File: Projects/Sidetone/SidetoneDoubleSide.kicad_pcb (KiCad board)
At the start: 2 copper layers, 109.1 x 105 mm, 54 parts, among them Q1 2N3904, Q2 2N3904, Q3 2N3904, SW1 morse key, SW2 On/off, U1 4N35, U2 LM324, U3 LM386

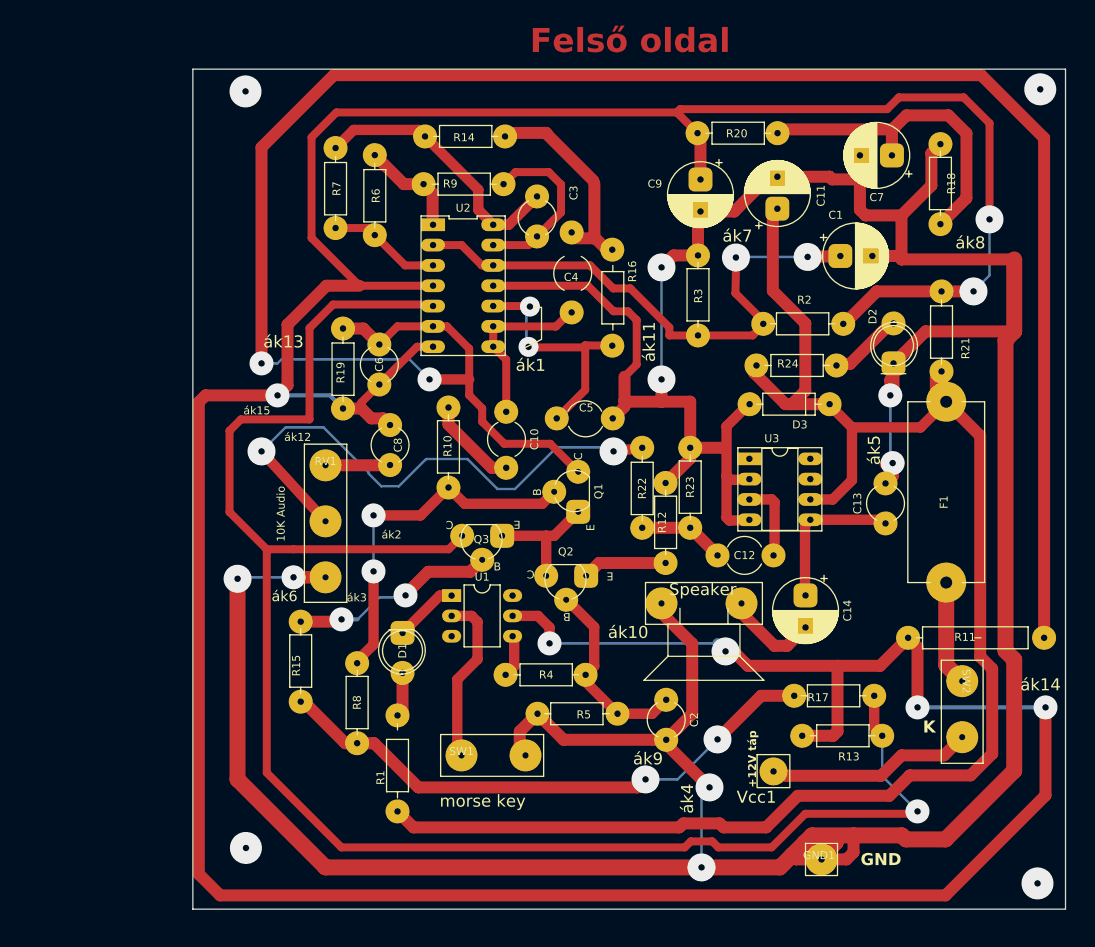
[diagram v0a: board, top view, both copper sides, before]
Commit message: 20240226
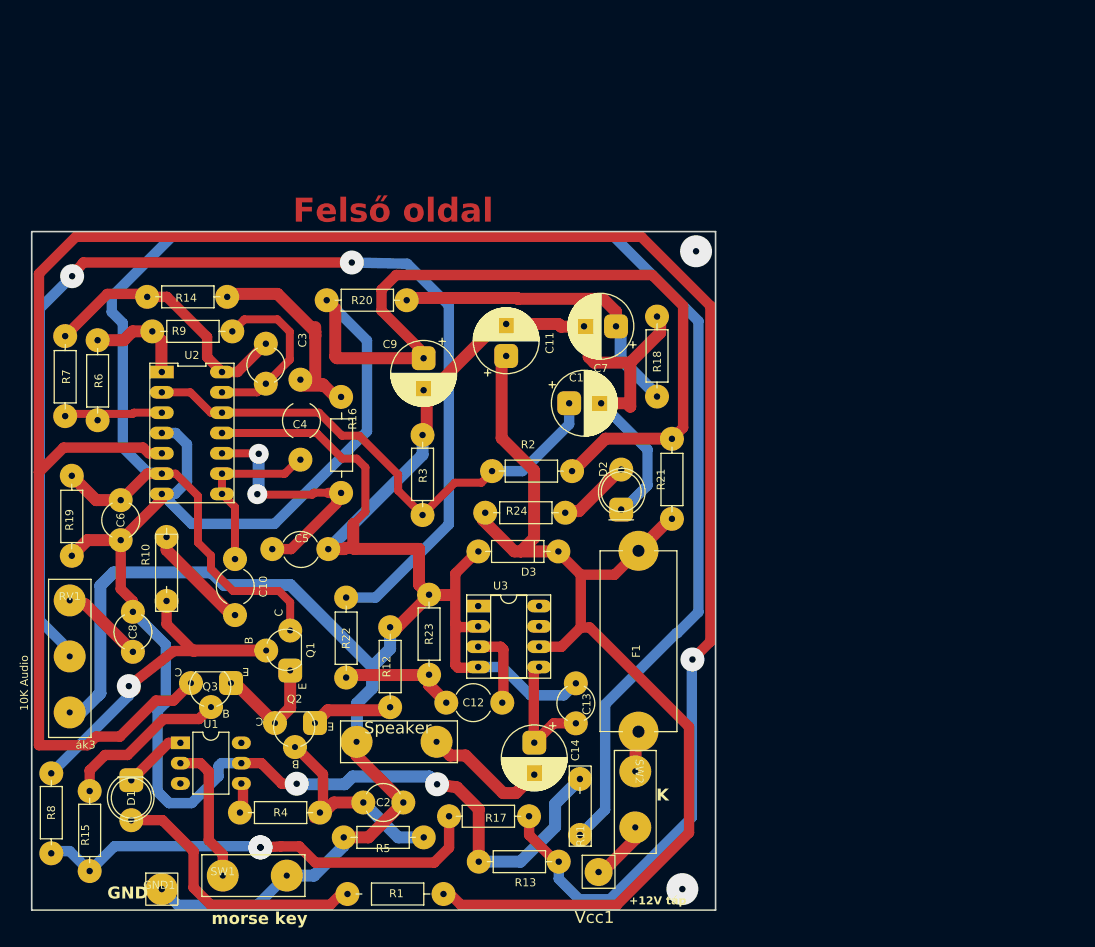
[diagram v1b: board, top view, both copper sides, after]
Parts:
- moved GND1 82.6 mm to (104.3, 144.8)
- moved R20 50.8 mm to (124.9, 71.1)
- moved C13 46.1 mm to (156.1, 124.0)
- moved R17 45.7 mm to (150.2, 135.7)
- moved R11 44.7 mm to (156.6, 131.0), turned to -90 degrees
- moved R13 43.4 mm to (143.9, 141.3)
- moved F1 42.7 mm to (163.9, 102.5)
- moved SW2 42.4 mm to (163.5, 130.0)
- moved 4-8ohm1 41.9 mm to (138.7, 126.3)
- moved R6 41.7 mm to (96.3, 76.1)
- moved R22 41.5 mm to (127.3, 108.3)
- moved R18 41.5 mm to (166.2, 83.2)
- moved C9 41.2 mm to (137.0, 78.4)
- moved R7 41.2 mm to (92.2, 75.6)
- moved Q1 41.1 mm to (120.4, 117.4)
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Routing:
- net Net-(U2E-V+): track 503.7 -> 288.1 mm, vias 7 -> 2
- net GNDD: track 500.4 -> 307.6 mm, vias 8 -> 0
- net Net-(R22-Pad1): track 70.7 -> 145.2 mm
- net Net-(Q3-C): track 212.9 -> 284.5 mm
- net Net-(D3-K): track 199.6 -> 139.0 mm
- net Net-(Q1-C): track 265.7 -> 221.6 mm, vias 2 -> 0
- net Net-(D1-A): track 5.57 -> 35.0 mm
- net VCC: track 25.8 -> 7.76 mm
- net Net-(R15-Pad1): track 70.9 -> 58.1 mm
- net Net-(SW2A-A): track 13.2 -> 5.14 mm
- net Net-(Q3-B): track 26.8 -> 21.0 mm, vias 2 -> 0
- net Net-(U2A--): track 70.2 -> 66.1 mm, vias 2 -> 0
- net Net-(C12-Pad1): track 10.9 -> 14.9 mm
- net Net-(4-8ohm1-Pad1): track 11.8 -> 15.8 mm
- net Net-(SW1A-A): track 21.5 -> 17.7 mm
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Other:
- board size 109.1 x 105 mm -> 85.5 x 84.8 mm
- board text added: "morse key"
- board text removed: "ák1"
- board text removed: "ák10"
- board text removed: "ák11"
- board text removed: "ák12"
- board text removed: "ák13"
- board text removed: "ák14"
- board text removed: "ák15"
- board text removed: "ák2"
- board text removed: "ák4"
- board text removed: "ák5"
- board text removed: "ák6"
- board text removed: "ák7"
- board text removed: "ák8"
- board text removed: "ák9"
